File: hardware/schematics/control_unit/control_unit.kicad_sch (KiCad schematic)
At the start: 5 parts, among them J1 Screw_Terminal_01x04, J2 Screw_Terminal_01x12, J3 Screw_Terminal_01x12, J4 6P6C

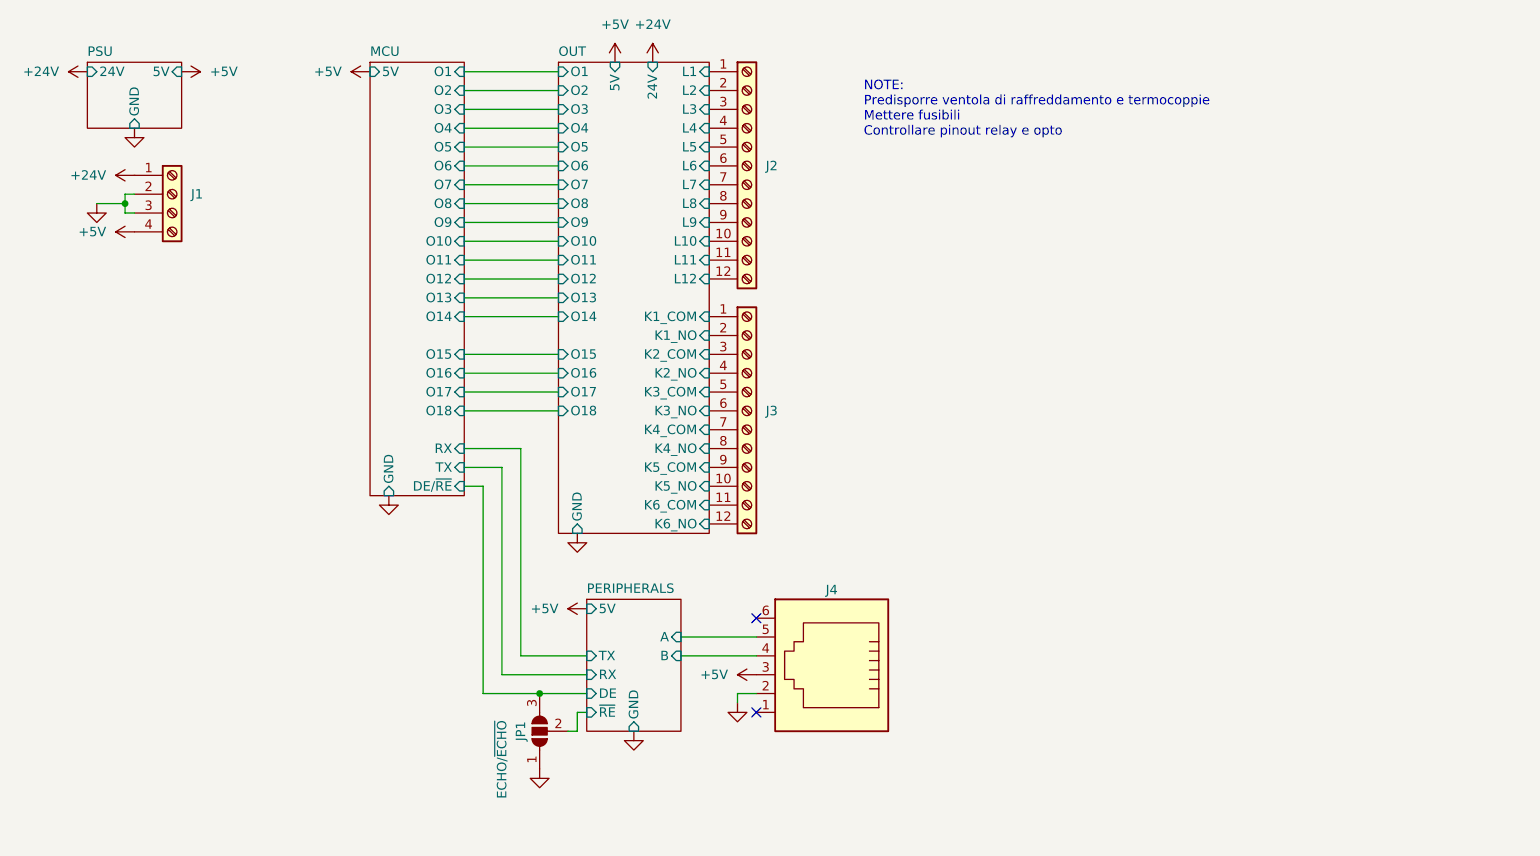
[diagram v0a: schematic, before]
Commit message: !feat
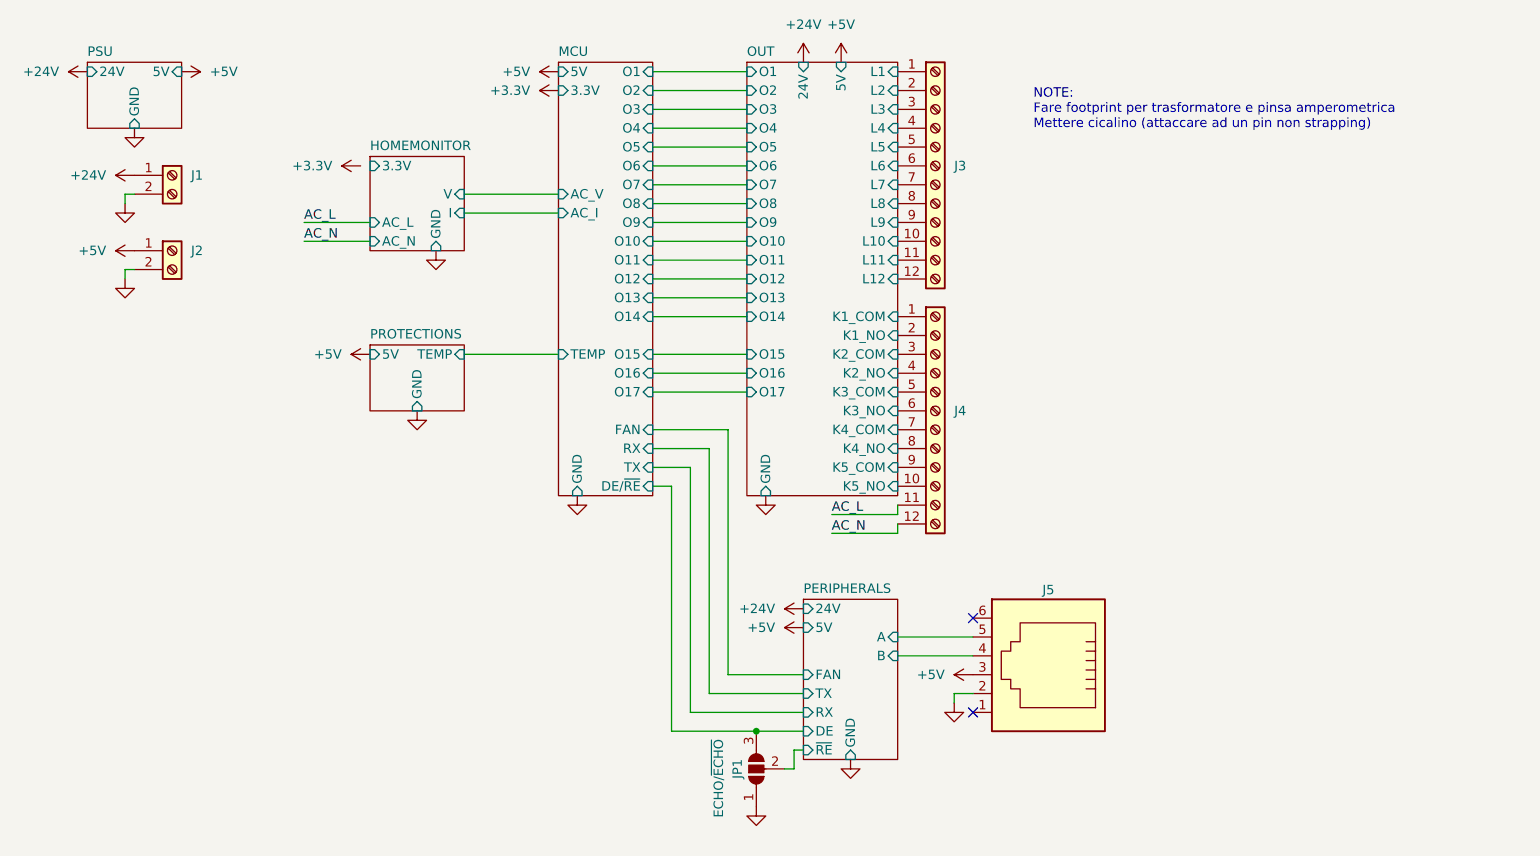
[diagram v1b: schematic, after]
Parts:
- removed J1: Screw_Terminal_01x04, symbol Connector:Screw_Terminal_01x04
- added J1, J2: Screw_Terminal_01x02, symbol Connector:Screw_Terminal_01x02
- renumbered J2 to J3, J3 to J4, J4 to J5
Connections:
- net +24V: now also J1.1 (Pin_1)
- net +5V: now also J2.1 (Pin_1)
- net GND: now also J1.2 (Pin_2), J2.2 (Pin_2)
- net OUT/K6_COM renamed AC_L
- net OUT/K6_NO renamed AC_N
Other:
- added sheet HOMEMONITOR (untitled.kicad_sch)
- added sheet PROTECTIONS (protections.kicad_sch)
- sheet MCU ports: added 3.3V, AC_I, AC_V, FAN, TEMP; removed O18
- sheet OUT ports: added none; removed K6_COM, K6_NO, O18
- sheet PERIPHERALS ports: added 24V, FAN; removed none
- note added: "NOTE: Fare footprint per trasformatore e pinsa amperometrica Mettere cicalino (attaccare ad un pin non strapping)"
- note removed: "NOTE: Predisporre ventola di raffreddamento e termocoppie Mettere fusibili Controllare pinout relay e opto"
- moved on the sheet: J3, J4, J5, JP1
